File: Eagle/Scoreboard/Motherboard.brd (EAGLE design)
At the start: 67.3 x 92.7 mm, 26 parts

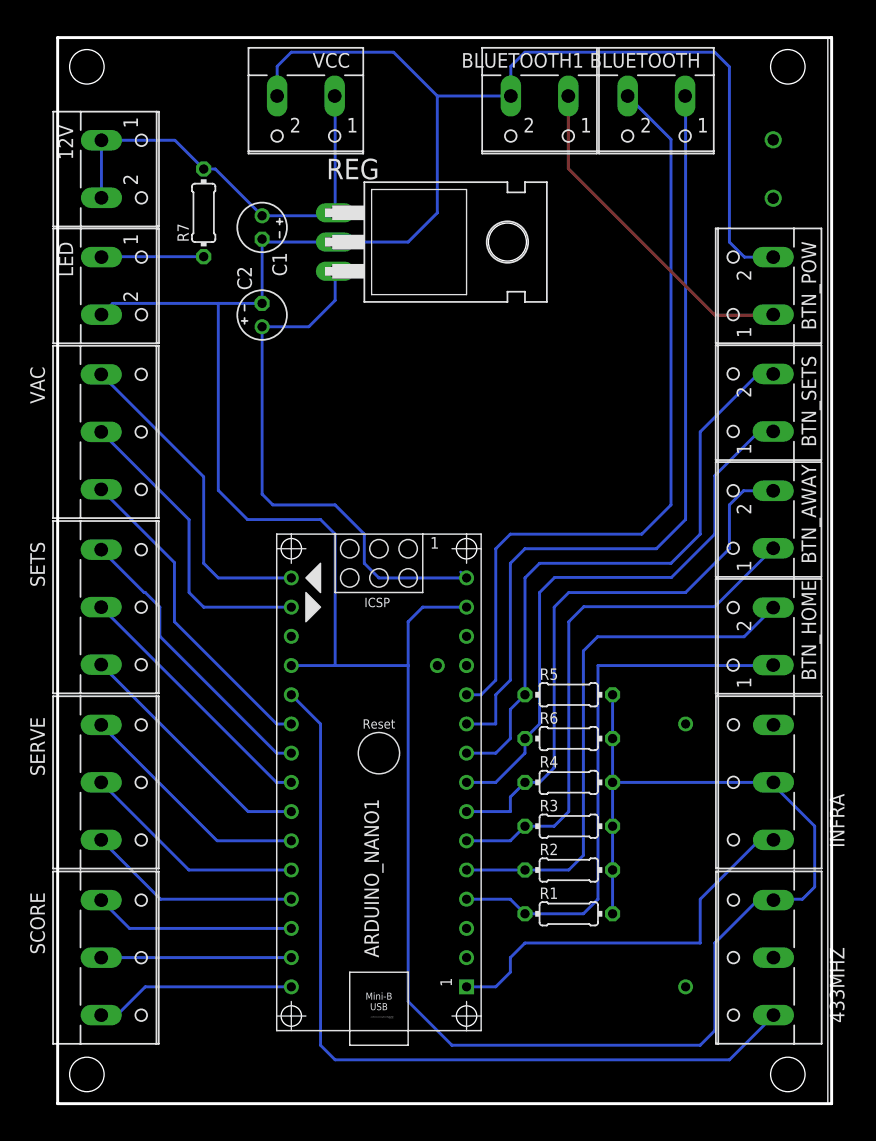
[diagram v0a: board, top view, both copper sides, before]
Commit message: Finalized board for motherboard
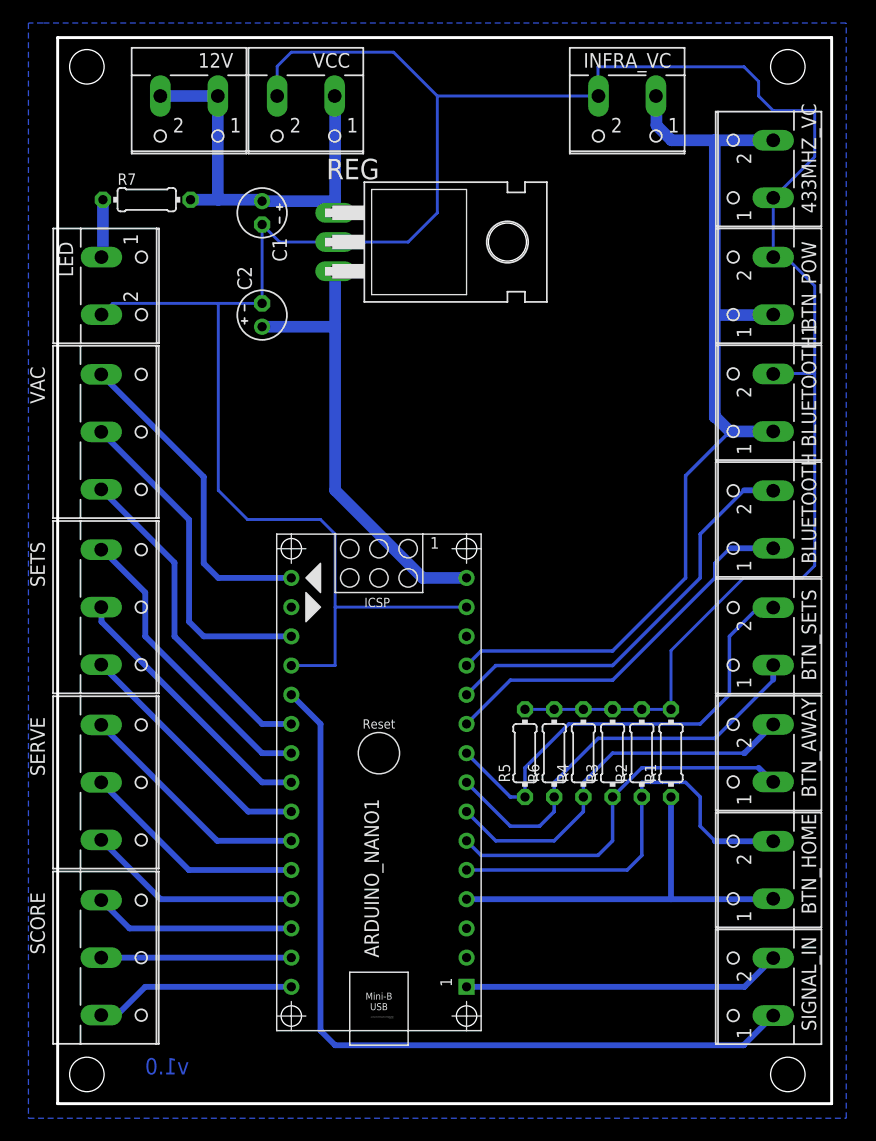
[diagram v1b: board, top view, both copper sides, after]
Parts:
- removed 433MHZ, INFRA: (no value), con-wago-500:W237-103
- added 433MHZ_VC, INFRA_VC, SIGNAL_IN: (no value), con-wago-500:W237-102
- moved BLUETOOTH 36.7 mm to (61.0, 50.8), turned to 90 degrees
- moved BLUETOOTH1 31.8 mm to (61.0, 61.0), turned to 90 degrees
- moved BTN_HOME 20.3 mm to (61.0, 20.3)
- moved BTN_SETS 20.3 mm to (61.0, 40.6)
- moved BTN_AWAY 20.3 mm to (61.0, 30.5)
- moved R1 16.6 mm to (53.3, 30.5), turned to 90 degrees
- moved R2 12.0 mm to (50.8, 30.5), turned to 90 degrees
- moved 12V 8.13 mm to (11.4, 86.4), turned to 180 degrees
- moved R3 7.41 mm to (48.3, 30.5), turned to 90 degrees
- moved R5 6.35 mm to (40.6, 30.5), turned to 90 degrees
- moved R7 5.08 mm to (7.75, 78.6), turned to 0 degrees
- moved R4 2.84 mm to (45.7, 30.5), turned to 90 degrees
- moved R6 1.80 mm to (43.2, 30.5), turned to 90 degrees
- moved C1 1.27 mm to (17.8, 77.5)
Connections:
- net N$10 renamed SCORE_3
- net N$11 renamed SCORE_2
- net N$12 renamed SCORE_1
- net N$13 renamed SERVE_3
- net N$14 renamed SERVE_2
- net N$15 renamed SERVE_1
- net N$16 renamed SETS_3
- net N$17 renamed SETS_2
- net N$18 renamed SETS_1
- net VIN renamed VIN_9V
- removed net VAC2: ARDUINO_NANO1.17, VAC.2
- new net RESET: ARDUINO_NANO1.18, VAC.2
- net 433MHZ: now also SIGNAL_IN.1; no longer 433MHZ.1
- net GND: now also 433MHZ_VC.1, INFRA_VC.2; no longer 433MHZ.3, INFRA.2
- net INFRA: now also SIGNAL_IN.2; no longer INFRA.1
- net VCC: now also 433MHZ_VC.2, INFRA_VC.1; no longer 433MHZ.2, INFRA.3
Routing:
- net VCC: track 30.7 -> 84.6 mm
- net GND: track 292.6 -> 239.6 mm
- net TXD: track 70.7 -> 33.7 mm
- net RXD: track 68.4 -> 36.3 mm
- net RESET: track 0.00 -> 29.1 mm
- net VAC2: track 26.6 -> 0.00 mm
- net N$4: track 49.4 -> 33.4 mm
- net N$5: track 51.0 -> 36.3 mm
- net N$3: track 46.9 -> 33.1 mm
- net N$6: track 53.0 -> 39.6 mm
- net N$1: track 48.1 -> 35.6 mm
- net N$2: track 46.5 -> 37.2 mm
- net INFRA: track 35.0 -> 27.7 mm
- net VIN_9V: track 47.4 -> 40.2 mm
- net N$7: track 8.96 -> 5.05 mm
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- added copper zone on layer 16, net GND
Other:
- outline, holes or cut-outs redrawn
- board text added: "v1.0"
